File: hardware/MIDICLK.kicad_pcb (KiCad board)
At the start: 2 copper layers, 20 x 110 mm, 32 parts, among them J1 Conn_02x06_Odd_Even, J2 AudioJack3, J3 AudioJack2, J4 AudioJack2, Q1 2N3904, Q2 2N3904, SW1 RotaryEncoder_Switch, U1 ATtiny85-20P, U2 6N138

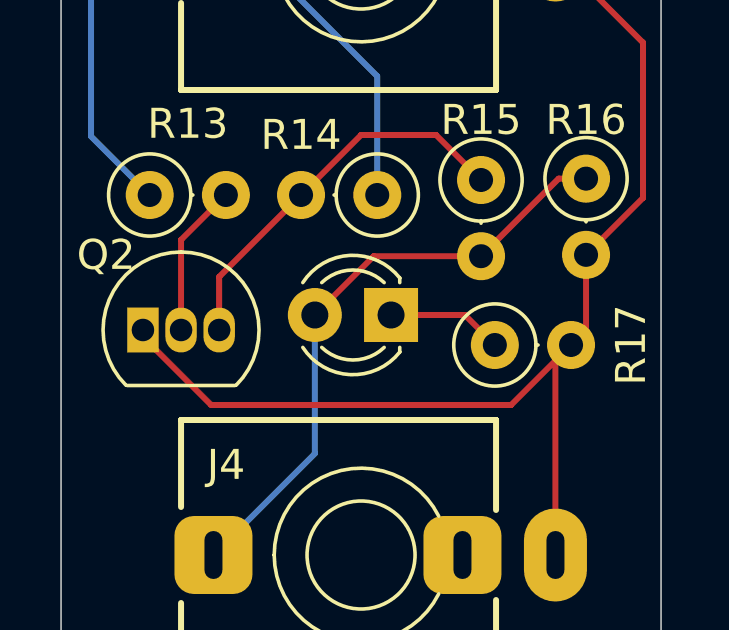
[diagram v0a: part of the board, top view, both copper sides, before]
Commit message: Add panel
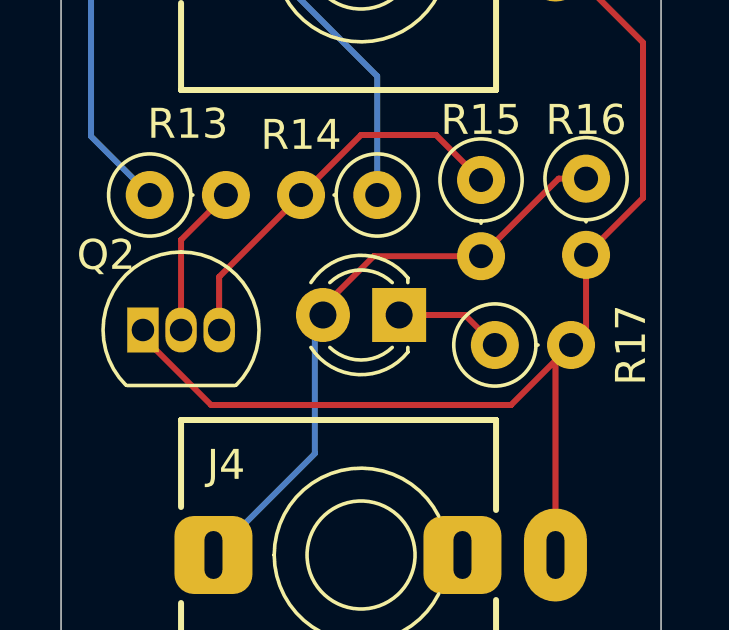
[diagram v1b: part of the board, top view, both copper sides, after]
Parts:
- moved D3 0.27 mm to (111.3, 115.5)
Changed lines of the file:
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@@
 	(footprint "LED_THT:LED_D3.0mm"
 		(layer "F.Cu")
-		(at 111 115.5 180)
+		(at 111.27 115.5 180)
 		(descr "LED, diameter 3.0mm, 2 pins, generated by kicad-footprint-generator")
 		(tags "LED")
